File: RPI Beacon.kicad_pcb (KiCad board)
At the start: 2 copper layers, 75 x 127 mm, 41 parts, among them J1 USB_C_Receptacle_PowerOnly_6P, Q1 FS8205A, SW1 SW_SPDT, U1 MCP73831-2-OT, U2 DW01A

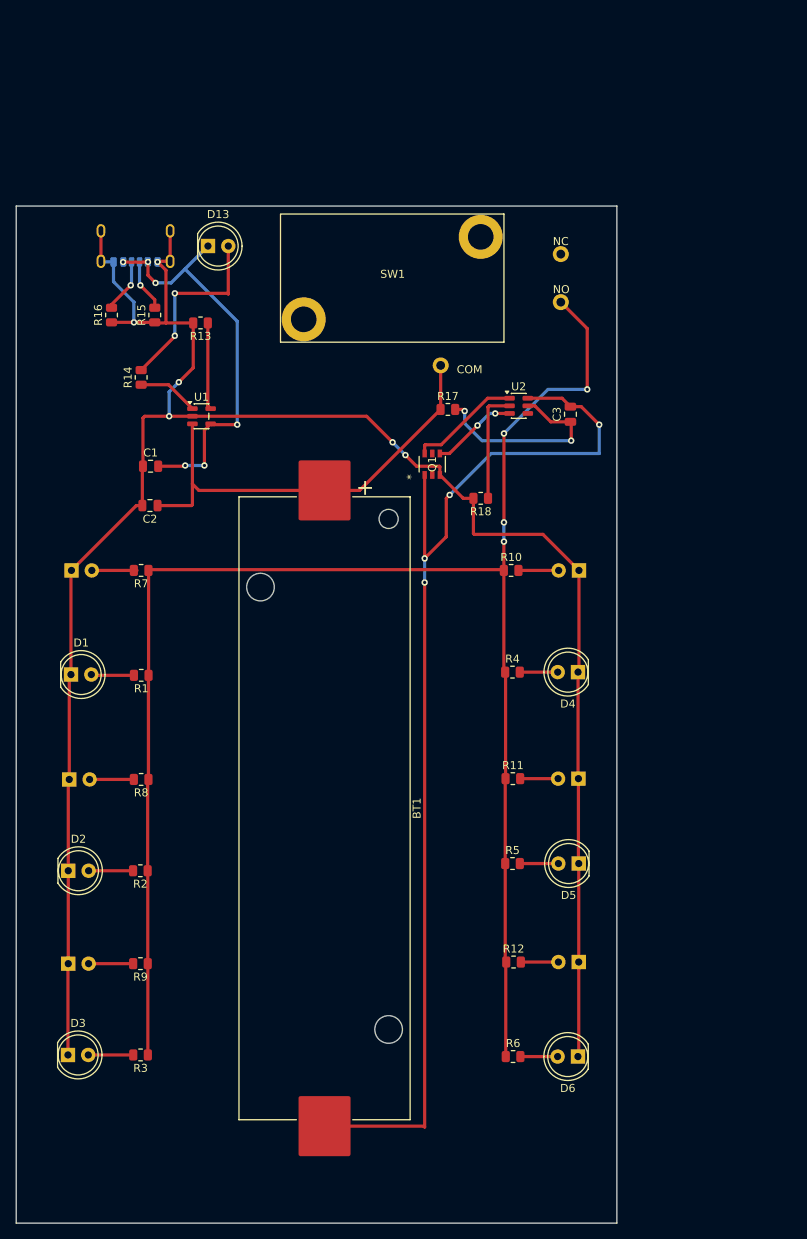
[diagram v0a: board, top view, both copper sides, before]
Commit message: minor revisions
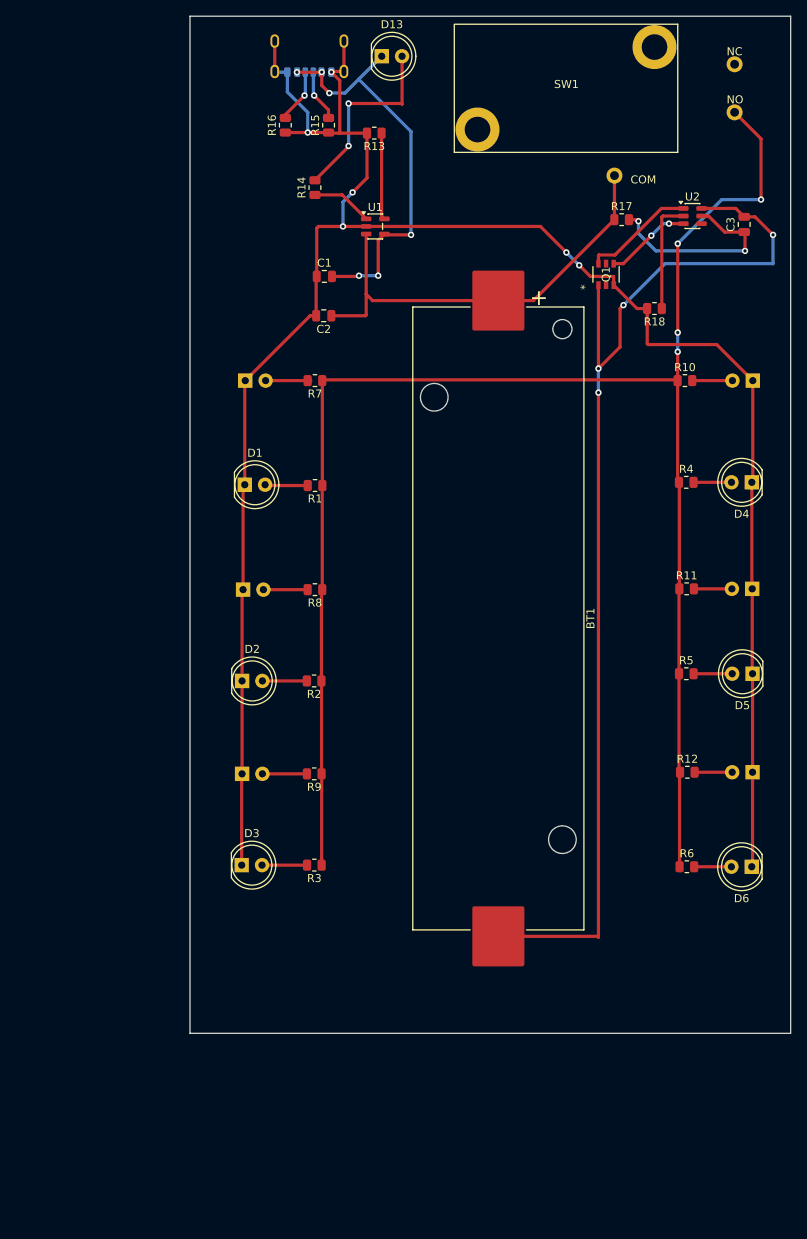
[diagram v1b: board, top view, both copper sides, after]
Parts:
- moved C3 32.1 mm to (160.9, 52.3)
- moved D11 32.1 mm to (161.9, 97.8)
- moved R11 32.1 mm to (153.7, 97.8)
- moved R12 32.1 mm to (153.8, 120.7)
- moved C2 32.1 mm to (108.4, 63.7)
- moved D2 32.1 mm to (98.2, 109.3)
- moved Q1 32.1 mm to (143.7, 58.5)
- moved R14 32.1 mm to (107.3, 47.7)
- moved R2 32.1 mm to (107.2, 109.3)
- moved R7 32.1 mm to (107.3, 71.8)
- moved U1 32.1 mm to (114.8, 52.5)
- moved D13 32.1 mm to (115.6, 31.3)
- moved D3 32.1 mm to (98.2, 132.3)
- moved D6 32.1 mm to (161.8, 132.5)
- moved D8 32.1 mm to (98.3, 97.9)
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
